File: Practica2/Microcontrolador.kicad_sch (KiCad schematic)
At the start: 8 parts, among them U2 ATtiny3216-S

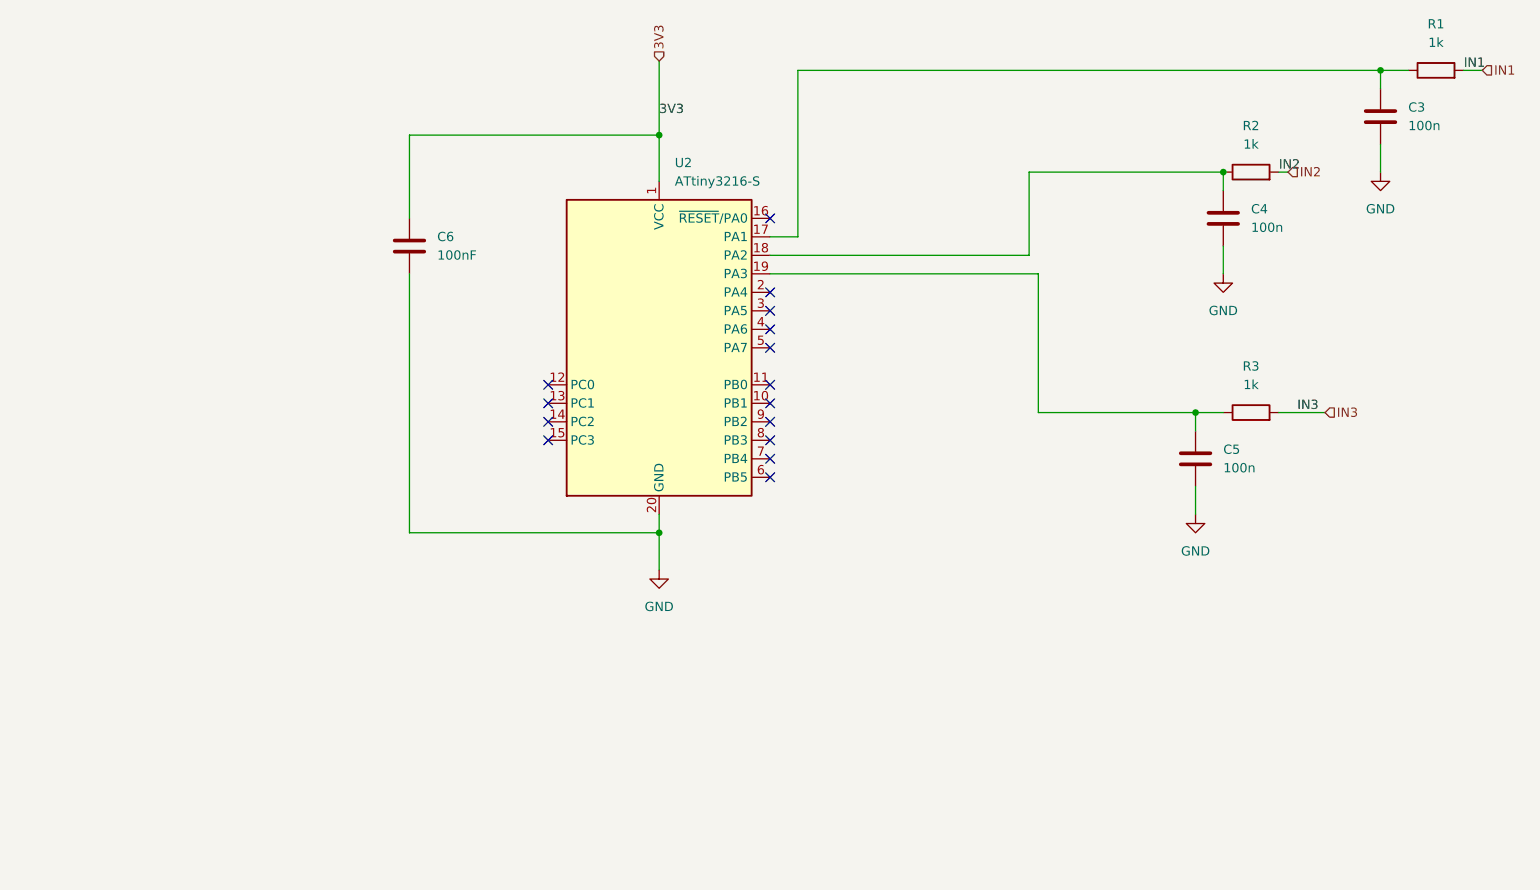
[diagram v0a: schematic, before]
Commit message: Actualización P4
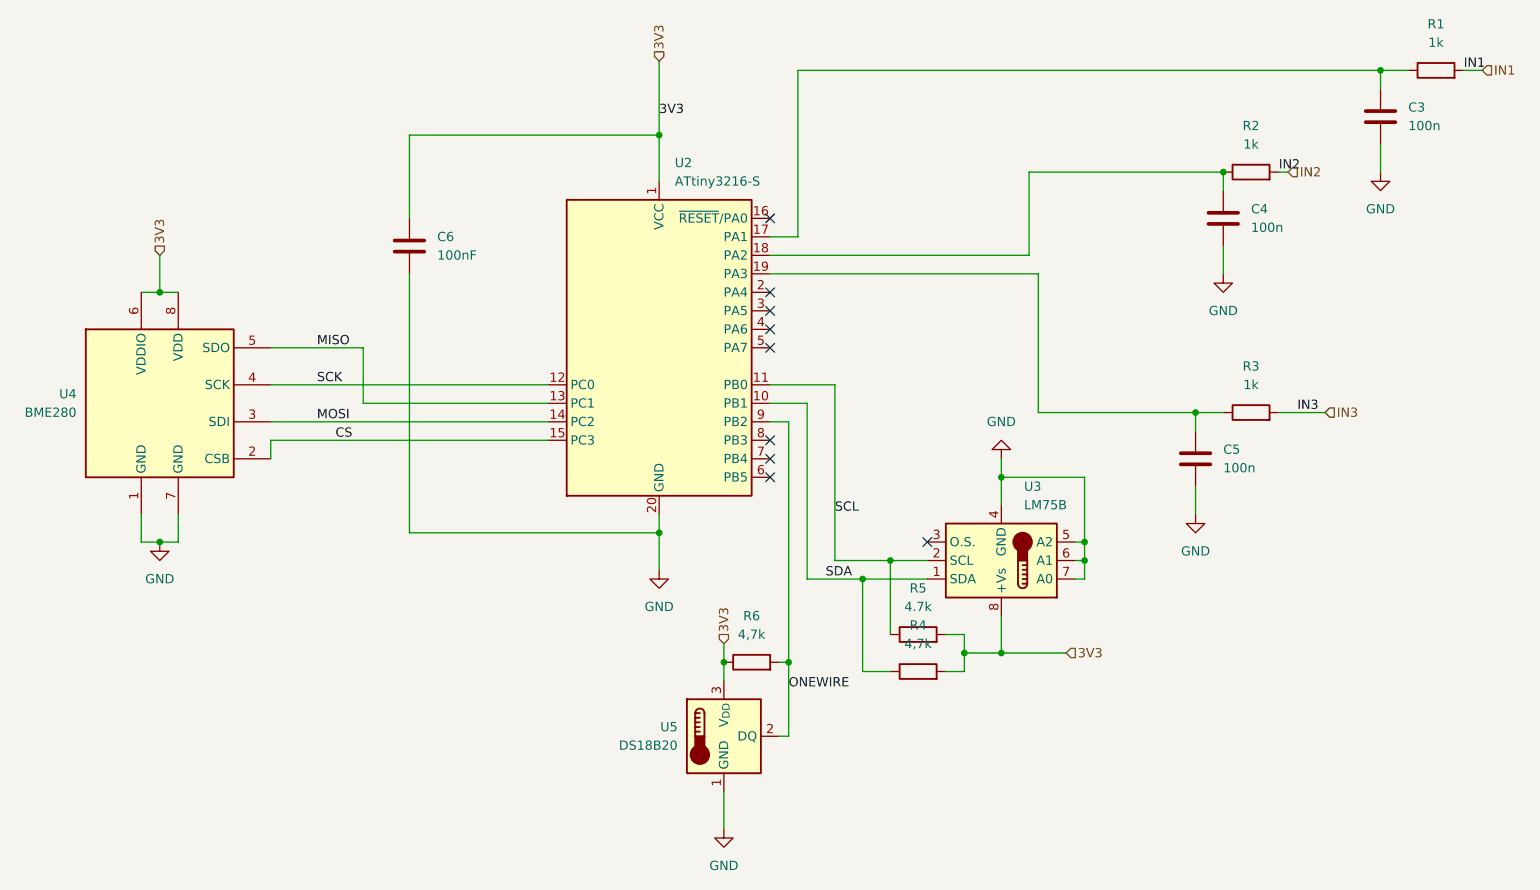
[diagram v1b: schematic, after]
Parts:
- added R4, R6: 4,7k, Resistor_SMD:R_0603_1608Metric, symbol Device:R
- added R5: 4.7k, Resistor_SMD:R_0603_1608Metric, symbol Device:R
- added U3: LM75B, Package_SO:VSSOP-8_2.3x2mm_P0.5mm, symbol Sensor_Temperature:LM75B
- added U4: BME280, Package_LGA:Bosch_LGA-8_2.5x2.5mm_P0.65mm_ClockwisePinNumbering, symbol Sensor:BME280
- added U5: DS18B20, Package_TO_SOT_THT:TO-92_Inline, symbol Sensor_Temperature:DS18B20
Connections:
- net 3V3: now also R4.2, R5.2, R6.1, U3.8 (+Vs), U4.6 (VDDIO), U4.8 (VDD), U5.3 (V_{DD})
- net GND: now also U3.4 (GND), U3.5 (A2), U3.6 (A1), U3.7 (A0), U4.1 (GND), U4.7 (GND), U5.1 (GND)
- net SDA: now reaches U2.10 (PB1)
- net SDA: now also R4.1, U3.1 (SDA)
- net SCL: now reaches U2.11 (PB0)
- net SCL: now also R5.1, U3.2 (SCL)
- net SCK: now reaches U2.12 (PC0)
- net SCK: now also U4.4 (SCK)
- net MISO: now reaches U2.13 (PC1)
- net MISO: now also U4.5 (SDO)
- net MOSI: now reaches U2.14 (PC2)
- net MOSI: now also U4.3 (SDI)
- net CS: now reaches U2.15 (PC3)
- net CS: now also U4.2 (CSB)
- net ONEWIRE: now reaches U2.9 (PB2)
- net ONEWIRE: now also R6.2, U5.2 (DQ)
- no-connect marks 15 -> 9
